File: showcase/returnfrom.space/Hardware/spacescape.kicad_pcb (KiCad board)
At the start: 4 copper layers, 195 x 120 mm, 313 parts, among them J1 USB_C_Receptacle_USB2.0_16P, J15 Conn_02x04_Odd_Even, J19 Conn_01x08_Pin, J2 Conn_01x08_Socket, J20 Conn_01x08_Socket, J21 Conn_01x08_Socket, J22 USB_C_Receptacle_USB2.0_16P, J23 USB_C_Receptacle_USB2.0_16P, J24 Conn_02x04_Odd_Even, J25 Conn_01x02, J26 Conn_02x07_Counter_Clockwise, J27 Conn_01x02, J3 OLED, J4 Conn_02x04_Odd_Even, J5 Conn_02x04_Odd_Even, J6 OLED, J7 OLED, Q1 Crystal_GND24, Q2 NPN, Q3 NPN, Q4 NPN, Q5 NPN, SW0 SW_SPST, SW1 SW_SPST, SW10 SW_SPST, SW11 SW_SPST, SW12 SW_SPST, SW13 SW_SPST, SW14 SW_SPST, SW15 SW_SPST, SW16 SW_SPST, SW17 RESET, SW18 BOOTSEL, SW19 SW_SPST, SW2 SW_SPST, SW20 SW_SPST, SW21 SW_SPST, SW22 SW_SPST, SW23 SW_SPDT_321, SW24 SW_SPDT_321, SW25 BOOTSEL, SW26 SW_SPST, SW27 SW_SPST, SW28 SW_SPST, SW29 SW_SPST, SW3 SW_SPST, SW30 SW_SPST, SW31 SW_SPST, SW32 SW_SPST, SW33 SW_SPST, SW34 SW_SPST, SW35 SW_SPDT_321, SW36 BOOTSEL, SW37 BOOTSEL, SW4 SW_SPST, SW5 SW_SPST, SW6 SW_SPST, SW7 SW_SPST, SW8 SW_SPST, SW9 SW_SPST, U1 AMS1117-3.3, U10 TLV62565DBVx, U12 TP4056, U13 TLV62565DBVx, U14 FM8002, U15 LIS2DH, U2 ESP32-S2-MINI-1, U3 RP2040, U4 MT3608L, U5 LM324, U6 TP4056, U7 LIS2DH, U8 W25Q128JVS, U9 ESP32-S2-MINI-2

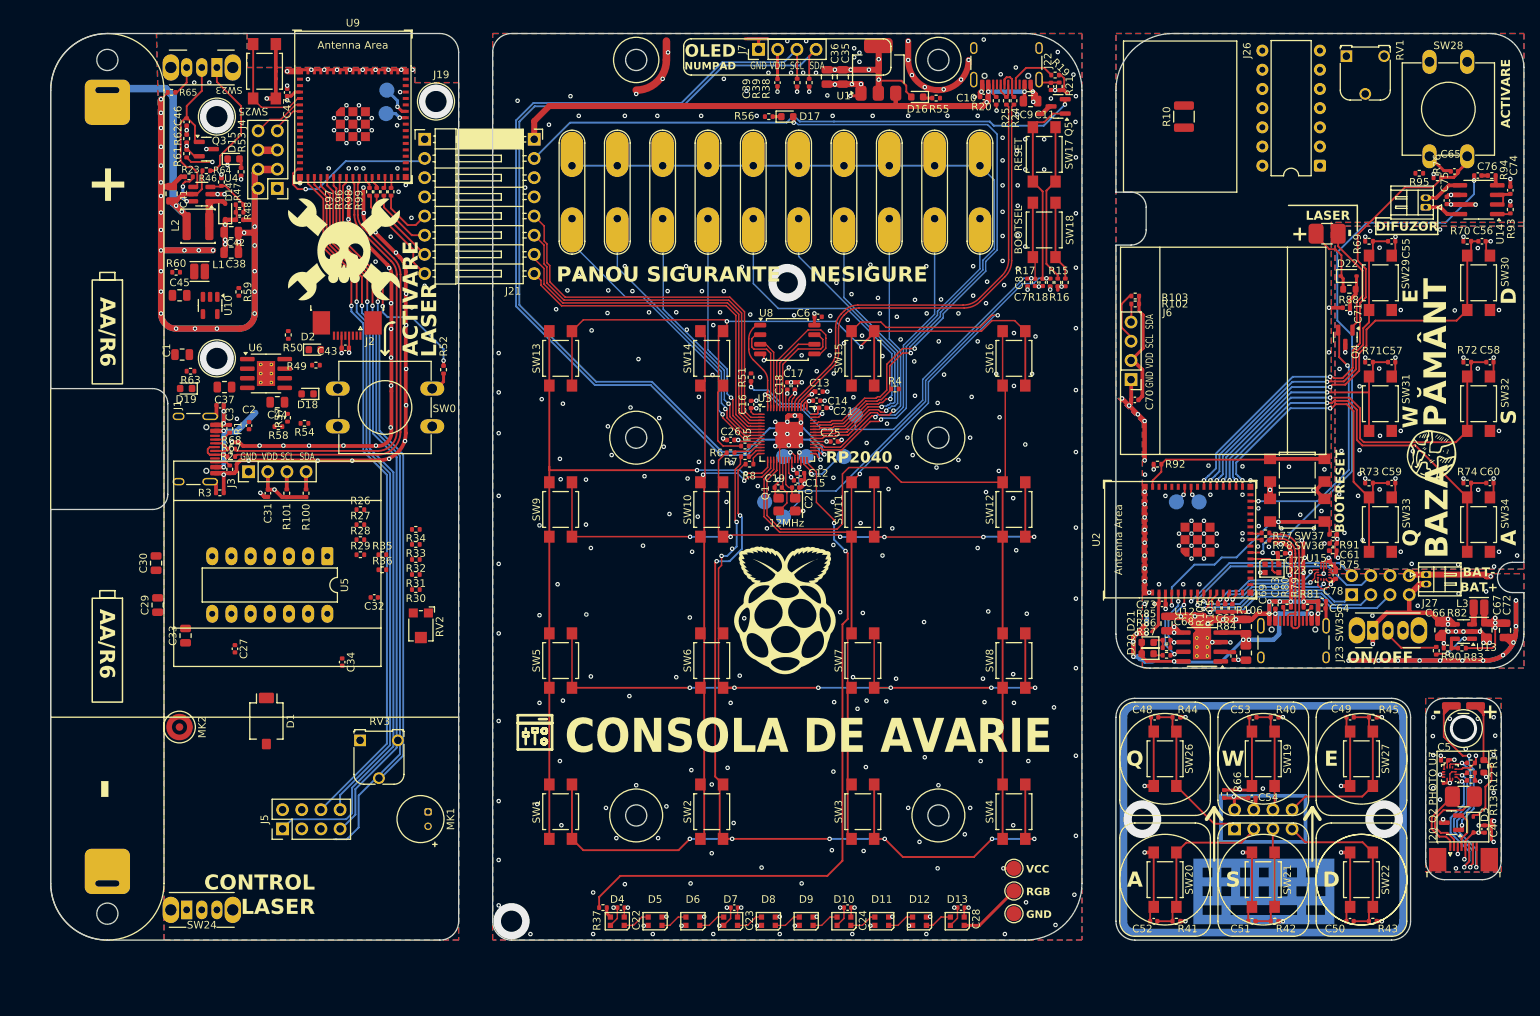
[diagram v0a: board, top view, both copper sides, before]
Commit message: panelizing...
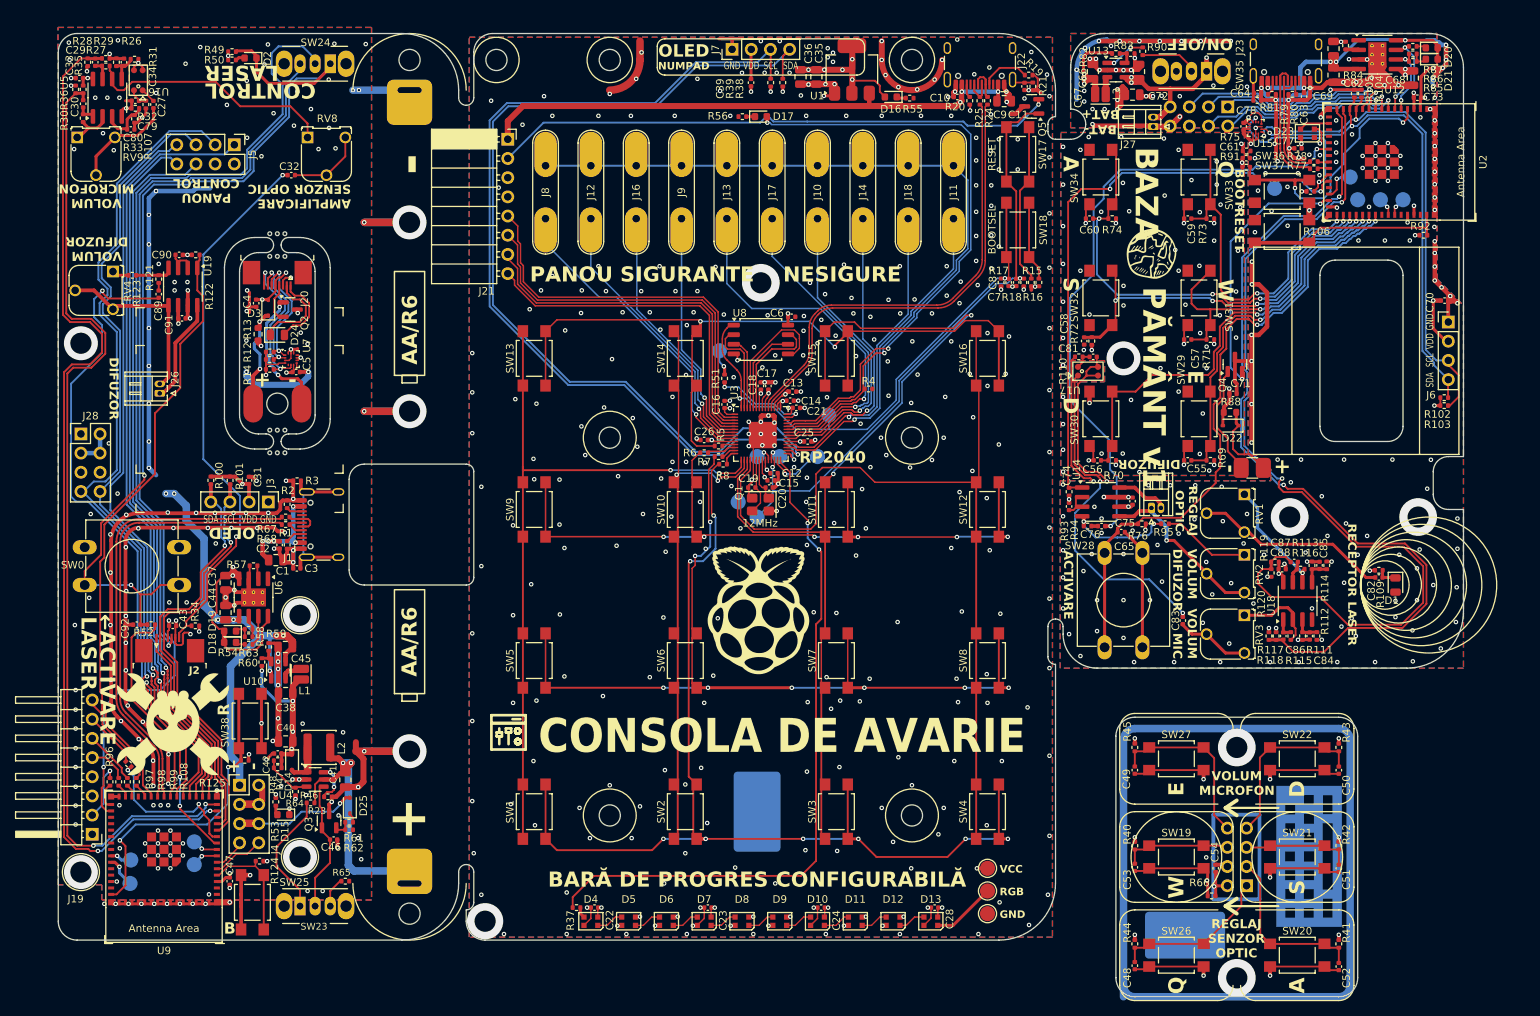
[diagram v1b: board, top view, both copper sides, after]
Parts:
- removed MK1: Microphone, Sensor_Audio:POM-2244P-C3310-2-R
- removed MK2: Microphone, Sensor_Audio:CUI_CMC-4013-SMT
- removed R10, R9: PHOTO, Resistor_SMD:R_1210_3225Metric
- added ADC3: TestPoint, TestPoint:TestPoint_Pad_D2.0mm, B.Cu at (108.5, 72.0)
- added AMP1: TestPoint, TestPoint:TestPoint_Pad_D2.0mm, B.Cu at (182.0, 50.5)
- added C79: 1uF, Capacitor_SMD:C_0402_1005Metric, F.Cu at (31.2, 38.9)
- added C80: 1uF, Capacitor_SMD:C_0402_1005Metric, F.Cu at (30.6, 42.7)
- added C81: 1uF, Capacitor_SMD:C_0402_1005Metric, F.Cu at (158.0, 72.8)
- added C82: 1uF, Capacitor_SMD:C_0402_1005Metric, F.Cu at (195.8, 102.0)
- added C83: 1uF, Capacitor_SMD:C_0402_1005Metric, F.Cu at (169.8, 107.7)
- added C84: 1uF, Capacitor_SMD:C_0402_1005Metric, F.Cu at (186.7, 109.8)
- added C85: 1uF, Capacitor_SMD:C_0402_1005Metric, F.Cu at (187.9, 100.4)
- added C86: 1uF, Capacitor_SMD:C_0402_1005Metric, F.Cu at (183.2, 109.8)
- added C87: 1uF, Capacitor_SMD:C_0402_1005Metric, F.Cu at (184.6, 100.0)
- added C88: 1uF, Capacitor_SMD:C_0402_1005Metric, F.Cu at (183.0, 100.9)
- added C89: 1uF, Capacitor_SMD:C_0402_1005Metric, F.Cu at (34.3, 64.5)
- added C90: 1uF, Capacitor_SMD:C_0402_1005Metric, F.Cu at (37.0, 59.3)
- added C91: 1uF, Capacitor_SMD:C_0402_1005Metric, F.Cu at (37.4, 67.7)
- added C92: 100nF, Capacitor_SMD:C_0402_1005Metric, F.Cu at (31.4, 108.2)
- added D24: TEMD7000X01, Diode_SMD:D_0805_2012Metric, F.Cu at (50.0, 69.9)
- added D25: D, Diode_SMD:D_SOD-323, F.Cu at (59.6, 132.2)
- added GND2: TestPoint, TestPoint:TestPoint_Pad_D2.0mm, B.Cu at (193.0, 52.0)
- added IO3: TestPoint, TestPoint:TestPoint_Pad_D2.0mm, B.Cu at (39.0, 140.0)
- added IO33: TestPoint, TestPoint:TestPoint_Pad_D2.0mm, B.Cu at (192.0, 49.0)
- added IO4: TestPoint, TestPoint:TestPoint_Pad_D2.0mm, B.Cu at (39.0, 137.0)
- added J28: Conn_02x04_Odd_Even, Connector_PinHeader_2.54mm:PinHeader_2x04_P2.54mm_Vertical, F.Cu at (24.0, 83.0)
- added R107: 1K, Resistor_SMD:R_0402_1005Metric, F.Cu at (32.6, 39.4)
- added R108: 27R, Resistor_SMD:R_0402_1005Metric, F.Cu at (27.9, 129.1)
- added R109: 47K, Resistor_SMD:R_0402_1005Metric, F.Cu at (195.8, 101.0)
- added R110: 1K, Resistor_SMD:R_0402_1005Metric, F.Cu at (156.1, 72.8)
- added R111: 47K, Resistor_SMD:R_0402_1005Metric, F.Cu at (185.7, 109.8)
- added R112: 47K, Resistor_SMD:R_0402_1005Metric, F.Cu at (187.6, 109.8)
- added R113: 47K, Resistor_SMD:R_0402_1005Metric, F.Cu at (186.9, 100.4)
- added R114: 47K, Resistor_SMD:R_0402_1005Metric, F.Cu at (188.9, 100.4)
- added R115: 47K, Resistor_SMD:R_0402_1005Metric, F.Cu at (184.2, 109.8)
- added R116: 47K, Resistor_SMD:R_0402_1005Metric, F.Cu at (185.4, 100.9)
- added R117: 47K, Resistor_SMD:R_0402_1005Metric, F.Cu at (181.2, 109.8)
- added R118: 47K, Resistor_SMD:R_0402_1005Metric, F.Cu at (182.2, 109.8)
- added R119: 47K, Resistor_SMD:R_0402_1005Metric, F.Cu at (182.1, 100.0)
- added R120: 47K, Resistor_SMD:R_0402_1005Metric, F.Cu at (181.6, 101.4)
- added R121: 5K1, Resistor_SMD:R_0402_1005Metric, F.Cu at (34.3, 62.5)
- added R122: 47K, Resistor_SMD:R_0402_1005Metric, F.Cu at (39.2, 59.3)
- added R123: 1K, Resistor_SMD:R_0402_1005Metric, F.Cu at (30.8, 62.0)
- added R124: 5K1, Resistor_SMD:R_0402_1005Metric, F.Cu at (47.6, 139.6)
- added R125: 5K1, Resistor_SMD:R_0402_1005Metric, F.Cu at (45.7, 126.2)
- added RV2: R_Potentiometer, Potentiometer_THT:Potentiometer_Runtron_RM-065_Vertical, F.Cu at (178.0, 99.0)
- added RV4: R_Potentiometer, Potentiometer_THT:Potentiometer_Runtron_RM-065_Vertical, F.Cu at (28.2, 61.5)
- added RV8: R_Potentiometer, Potentiometer_THT:Potentiometer_Runtron_RM-065_Vertical, F.Cu at (54.0, 43.8)
- added SW38: RESET, Button_Switch_SMD:SW_SPST_TL3305C, F.Cu at (46.4, 121.0)
- added U16: LMA3722T421-OA5, spacescape:LMA3722T421, F.Cu at (31.6, 36.2)
- added U17: LMA3722T421-OA5, spacescape:LMA3722T421, F.Cu at (157.3, 74.7)
- added U18: TLV2372, Package_SO:SOIC-8_3.9x4.9mm_P1.27mm, F.Cu at (185.1, 105.1)
- added U19: FM8002, Package_SO:SOIC-8_3.9x4.9mm_P1.27mm, F.Cu at (37.5, 63.5)
- C27, C34: value 100n -> 1uF
- C29, C30, C33: value 22uF -> 1uF; footprint Capacitor_SMD:C_0805_2012Metric -> Capacitor_SMD:C_0402_1005Metric
- C32: value 15pF -> 1uF
- D1: value BP104-SMD -> TEMD7000X01; footprint OptoDevice:Osram_BP104-SMD -> Diode_SMD:D_0805_2012Metric
- J10, J11, J12, J13, J14, J16, J17, J18, J8, J9: footprint spacescape:Untitled -> spacescape:RES-PAD
- J26: value Conn_02x07_Counter_Clockwise -> Conn_01x02; footprint Package_DIP:DIP-14_W7.62mm -> Connector_Hirose:Hirose_DF13-02P-1.25DS_1x02_P1.25mm_Horizontal
- R26, R27, R28: value 10k -> 47K
- R29: value 1k -> 47K
- R31, R34, R93: value 5K1 -> 47K
- R35, R36: value 100k -> 47K
- RV1, RV3: value R_Potentiometer_Trim -> R_Potentiometer
- RV9: renamed from RV2; footprint Potentiometer_SMD:Potentiometer_Bourns_TC33X_Vertical -> Potentiometer_THT:Potentiometer_Runtron_RM-065_Vertical
- SW37: value BOOTSEL -> RESET
- U5: value LM324 -> TLV2372; footprint Package_DIP:DIP-14_W7.62mm_LongPads -> Package_SO:SOIC-8_3.9x4.9mm_P1.27mm
- moved C4 176.9 mm to (47.2, 65.7), turned to -90 degrees
- moved J20 174.9 mm to (50.0, 62.0), turned to 180 degrees
- moved D3 173.5 mm to (48.8, 66.3), turned to 90 degrees
- moved R22 172.0 mm to (47.5, 69.8)
- moved R13 168.8 mm to (49.0, 72.2), turned to 0 degrees
- moved R12 168.1 mm to (49.0, 73.2), turned to 0 degrees
- moved Q2 168.0 mm to (51.7, 66.5), turned to 0 degrees
- moved R14 167.3 mm to (49.0, 74.5), turned to 0 degrees
- moved U7 162.9 mm to (51.8, 73.1), turned to 0 degrees
- moved R11 162.0 mm to (50.0, 79.0), turned to 180 degrees
- moved C5 160.5 mm to (52.5, 74.8), turned to 0 degrees
- moved J26 156.5 mm to (34.4, 77.6), turned to 90 degrees
- moved D1 150.5 mm to (198.0, 103.0)
- moved RV3 118.2 mm to (178.0, 107.0), turned to -90 degrees
- moved SW24 113.6 mm to (57.0, 34.0), turned to 180 degrees
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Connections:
- net /remote/RXD3 renamed /remote/RXD0
- net /remote/TXD3 renamed /remote/TXD0
- net Net-(J24-Pin_1) renamed /remote/IO5
- net Net-(J24-Pin_2) renamed /remote/IO3
- net Net-(J24-Pin_3) renamed /remote/IO6
- net Net-(J24-Pin_4) renamed /remote/IO4
- net Net-(J24-Pin_5) renamed /remote/IO7
- net Net-(SW1-A) renamed /numpad/IO12
- net Net-(SW10-A) renamed /numpad/IO13
- net Net-(SW11-A) renamed /numpad/IO14
- net Net-(SW12-A) renamed /numpad/IO15
- net Net-(U11-+3V) renamed +3V0
- net Net-(U3-GPIO10) renamed /numpad/IO10
- net Net-(U3-GPIO11) renamed /numpad/IO11
- net RGB renamed /numpad/RGB
- net RST1 renamed /numpad/RST1
- C27 pad 1: +5V -> Net-(U16-OUT)
- C27 pad 2: GND -> Net-(C27-Pad2)
- C29 pad 2: GND -> ADC1
- C30 pad 2: /amp/ADC -> ADC2
- C32 pad 1: Net-(U5B--) -> LDR
- C32 pad 2: Net-(C30-Pad1) -> Net-(C32-Pad2)
- C33 pad 1: Net-(MK2-+) -> GND
- C33 pad 2: Net-(U5B-+) -> +3V3
- C34 pad 1: Net-(MK2-+) -> +3V3
- C34 pad 2: GND -> Net-(U5B-+)
- C74 pad 1: GND -> Net-(U14-BYPS)
- C74 pad 2: Net-(U14-BYPS) -> GND
- J19 pad 2: /motherboard/IO11 -> /motherboard/IO35
- J19 pad 7: /motherboard/IO26 -> /motherboard/IO6
- J19 pad 8: /motherboard/IO21 -> /motherboard/IO26
- J2 pad 1: ACC_INT -> /motherboard/INT2
- J2 pad 2: SDA -> /motherboard/SDA2
- J2 pad 3: SCL -> /motherboard/SCL2
- J2 pad 5: Net-(D2-K) -> Net-(J2-Pin_5)
- J2 pad 7: PHOTO1 -> LDR
- J2 pad 8: PHOTO2 -> GND
- J26 pad 1: unconnected-(J26-Pin_1-Pad1) -> Net-(J26-Pin_1)
- J26 pad 2: unconnected-(J26-Pin_2-Pad2) -> Net-(J26-Pin_2)
- J3 pad 3: Net-(J3-Pin_3) -> /motherboard/SCL2
- J3 pad 4: Net-(J3-Pin_4) -> /motherboard/SDA2
- J4 pad 2: Net-(J4-Pin_2) -> GND
- J4 pad 3: Net-(J4-Pin_2) -> GND
- J5 pad 3: unconnected-(J5-Pin_3-Pad3) -> /motherboard/K6
- J5 pad 5: unconnected-(J5-Pin_5-Pad5) -> /motherboard/K5
- J5 pad 8: unconnected-(J5-Pin_8-Pad8) -> /motherboard/K2
- J6 pad 3: Net-(J6-Pin_3) -> /remote/SCL3
- J6 pad 4: Net-(J6-Pin_4) -> /remote/SDA3
- R100 pad 2: Net-(J3-Pin_4) -> /motherboard/SDA2
- R101 pad 1: Net-(J3-Pin_3) -> /motherboard/SCL2
- R102 pad 2: Net-(J6-Pin_4) -> /remote/SDA3
- R103 pad 1: Net-(J6-Pin_3) -> /remote/SCL3
- R26 pad 1: Net-(R26-Pad1) -> Net-(U5B--)
- R26 pad 2: +5V -> Net-(C29-Pad1)
- R27 pad 1: GND -> ADC1
- R27 pad 2: Net-(R27-Pad2) -> +3V3
- R28 pad 1: Net-(D1-K) -> GND
- R28 pad 2: +5V -> ADC1
- R29 pad 1: /amp/GPIO -> Net-(U5B-+)
- R29 pad 2: Net-(R29-Pad2) -> +3V3
- R30 pad 1: Net-(U5B--) -> Net-(U5A--)
- R31 pad 1: Net-(U5B--) -> Net-(U5B-+)
- R31 pad 2: Net-(C29-Pad1) -> GND
- R32 pad 1: Net-(U5B-+) -> Net-(U5A-+)
- R33 pad 1: Net-(U5B-+) -> Net-(U5A-+)
- R34 pad 2: Net-(MK2-+) -> LDR
- R35 pad 1: /amp/ADC -> ADC2
- R36 pad 2: /amp/ADC -> ADC2
- R51 pad 2: unconnected-(R51-Pad2) -> Net-(ADC3-Pad1)
- R52 pad 1: Net-(SW0-A) -> Net-(D2-K)
- R61 pad 2: +5V -> Net-(D25-K)
- R93 pad 1: +3V3 -> GND
- R93 pad 2: Net-(U14-SHDN) -> /remote/AMP_EN
- R95 pad 1: GND -> Net-(U14-IN-)
- R96 pad 1: Net-(U9-SPI_CS1/GPIO26) -> /motherboard/IO6
- R96 pad 2: /motherboard/IO26 -> Net-(U9-GPIO6/ADC1_CH5)
- R97 pad 1: /motherboard/IO21 -> /motherboard/IO26
- R97 pad 2: Net-(U9-GPIO21) -> Net-(U9-SPI_CS1/GPIO26)
- RV1 pad 1: Net-(J25-Pin_2) -> Net-(U18B--)
- RV1 pad 2: Net-(J25-Pin_2) -> Net-(C82-Pad2)
- RV1 pad 3: Net-(R95-Pad2) -> Net-(C82-Pad2)
- RV3 pad 1: unconnected-(RV3-Pad1) -> Net-(U18A--)
- RV3 pad 2: unconnected-(RV3-Pad2) -> Net-(C83-Pad2)
- RV3 pad 3: unconnected-(RV3-Pad3) -> Net-(C83-Pad2)
- RV9 pad 1: Net-(R26-Pad1) -> Net-(U5A--)
- RV9 pad 2: Net-(U5A-+) -> Net-(C27-Pad2)
- RV9 pad 3: Net-(R27-Pad2) -> Net-(C27-Pad2)
- SW0 pad 1: Net-(SW0-A) -> Net-(D2-K)
- SW24 pad 1: Net-(SW0-A) -> Net-(D2-K)
- SW24 pad 2: Net-(D2-K) -> Net-(J2-Pin_5)
- SW24 pad 3: LASER_EN -> /motherboard/LASER_EN
- U14 pad 1: Net-(U14-SHDN) -> /remote/AMP_EN
- U14 pad 5: Net-(J25-Pin_2) -> Net-(J25-Pin_1)
- U14 pad 8: Net-(J25-Pin_1) -> Net-(J25-Pin_2)
- U2 pad 14: /remote/INT3 -> /remote/ADC1
- U2 pad 15: unconnected-(U2-GPIO11/ADC2_CH0-Pad15) -> /remote/ADC2
- U2 pad 17: unconnected-(U2-GPIO13/ADC2_CH2-Pad17) -> /remote/RGB
- U2 pad 20: /remote/RGB -> unconnected-(U2-GPIO16/ADC2_CH5/XTAL_32K_N-Pad20)
- U2 pad 25: unconnected-(U2-GPIO21-Pad25) -> /remote/INT3
- U2 pad 26: unconnected-(U2-SPI_CS1/GPIO26-Pad26) -> /remote/AMP_EN
- U2 pad 28: unconnected-(U2-GPIO33-Pad28) -> Net-(U2-GPIO33)
- U5 pad 1: Net-(R29-Pad2) -> Net-(C30-Pad1)
- U5 pad 2: Net-(D1-K) -> Net-(U5A--)
- U5 pad 4: +5V -> GND
- U5 pad 7: Net-(C30-Pad1) -> Net-(C29-Pad1)
- U5 pad 8: unconnected-(U5-Pad8) -> +3V3
- U9 pad 10: unconnected-(U9-GPIO6/ADC1_CH5-Pad10) -> Net-(U9-GPIO6/ADC1_CH5)
- U9 pad 11: unconnected-(U9-GPIO7/ADC1_CH6-Pad11) -> /motherboard/SCL2
- U9 pad 12: unconnected-(U9-GPIO8/ADC1_CH7-Pad12) -> /motherboard/SDA2
- U9 pad 13: unconnected-(U9-GPIO9/ADC1_CH8-Pad13) -> /motherboard/INT2
- U9 pad 14: unconnected-(U9-GPIO10/ADC1_CH9-Pad14) -> ADC1
- U9 pad 15: /motherboard/IO11 -> ADC2
- U9 pad 21: /motherboard/K6 -> /motherboard/DAC1
- U9 pad 25: Net-(U9-GPIO21) -> /motherboard/AMP_EN
- U9 pad 31: unconnected-(U9-GPIO35-Pad31) -> Net-(U9-GPIO35)
- U9 pad 32: unconnected-(U9-GPIO36-Pad32) -> /motherboard/LASER_EN
- U9 pad 45: unconnected-(U9-CHIP/PU/RESET-Pad45) -> Net-(SW38-B)
- U9 pad 7: unconnected-(U9-GPIO3/ADC1_CH2-Pad7) -> Net-(U9-GPIO3/ADC1_CH2)
- U9 pad 8: unconnected-(U9-GPIO4/ADC1_CH3-Pad8) -> Net-(U9-GPIO4/ADC1_CH3)
- U9 pad 9: unconnected-(U9-GPIO5/ADC1_CH4-Pad9) -> /motherboard/K6
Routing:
- net GND: track 640.4 -> 805.7 mm, vias 560 -> 704
- net ADC1: track 0.00 -> 137.2 mm, vias 0 -> 2
- net ADC2: track 0.00 -> 130.8 mm, vias 0 -> 2
- net Net-(D2-K): track 0.00 -> 128.5 mm, vias 0 -> 2
- net /motherboard/LASER_EN: track 0.00 -> 124.2 mm, vias 0 -> 1
- net /remote/ADC1: track 0.00 -> 123.0 mm, vias 0 -> 2
- net /remote/ADC2: track 0.00 -> 114.4 mm, vias 0 -> 2
- net VBAT: track 79.6 -> 189.5 mm, vias 5 -> 13
- net Net-(J2-Pin_5): track 0.00 -> 104.6 mm, vias 0 -> 1
- net +5V: track 136.3 -> 223.7 mm, vias 11 -> 15
- net /motherboard/DAC1: track 0.00 -> 85.5 mm, vias 0 -> 2
- net /motherboard/AMP_EN: track 0.00 -> 80.6 mm
- net /remote/AMP_EN: track 0.00 -> 79.9 mm, vias 0 -> 2
- net LDR: track 0.00 -> 72.3 mm, vias 0 -> 2
- net /motherboard/SCL2: track 0.00 -> 56.2 mm, vias 0 -> 1
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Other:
- board size 195 x 120 mm -> 186 x 127.5 mm
- board text added: "+ -"
- board text added: "4V2"
- board text added: "6"
- board text added: "AMPLIFICARE SENZOR OPTIC"
- board text added: "B"
- board text added: "BARĂ DE PROGRES CONFIGURABILĂ"
- board text added: "CONTROL"
- board text added: "IO16"
- board text added: "IO4"
- board text added: "IO5"
- board text added: "M3"
- board text added: "M4"
- board text added: "OLED"
- board text added: "PANOU CONTROL"
- board text added: "PANOU CONTROL BAZA PAMÂNT"
- board text added: "PANOU CONTROL SIGMA"
- board text added: "PLACĂ BAZĂ SIGMA V1.0"
- board text added: "PĂMÂNT v1"
- board text added: "R"
- board text added: "RECEPTOR LASER"
- board text added: "REGLAJ OPTIC"
- board text added: "REGLAJ SENZOR OPTIC"
- board text added: "RFS"
- board text added: "RXD0"
- board text added: "SERVO"
- board text added: "TXD0"
- board text added: "VBAT"
- board text added: "VOLUM DIFUZOR"
- board text added: "VOLUM MIC"
- board text added: "VOLUM MICROFON"
- board text added: "a"
- board text added: "update de firmware pe returnfrom.space folosind thonny.org"
- board text added: "Σ"
- board text added: "Ω"
- board text removed: "CONTROL LASER"
- board text removed: "IO21"
- board text removed: "PANOU CONTROL DELTA"
- board text removed: "PLACĂ DE BAZĂ"
- board text removed: "PĂMÂNT"
- board text removed: "update de firmware thonny.org"
